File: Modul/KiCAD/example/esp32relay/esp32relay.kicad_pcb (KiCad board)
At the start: 2 copper layers, 49.7 x 53.8 mm, 22 parts, among them J1 Conn_01x03_Male, J2 Conn_01x02_Male, SW1 SW_Push, SW2 SW_Push, U1 ESP32-WROOM-32, U2 AMS1117-3.3

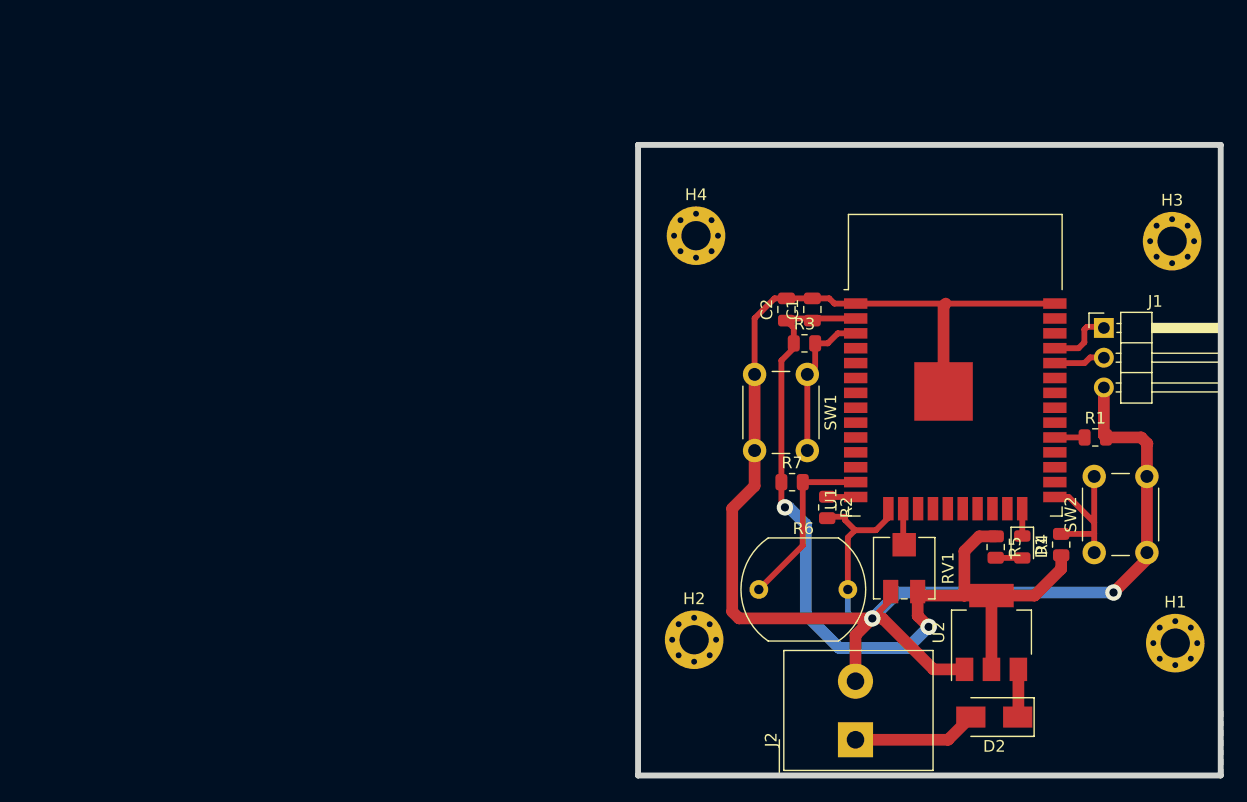
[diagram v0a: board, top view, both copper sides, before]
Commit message: KiCAD Fab Files
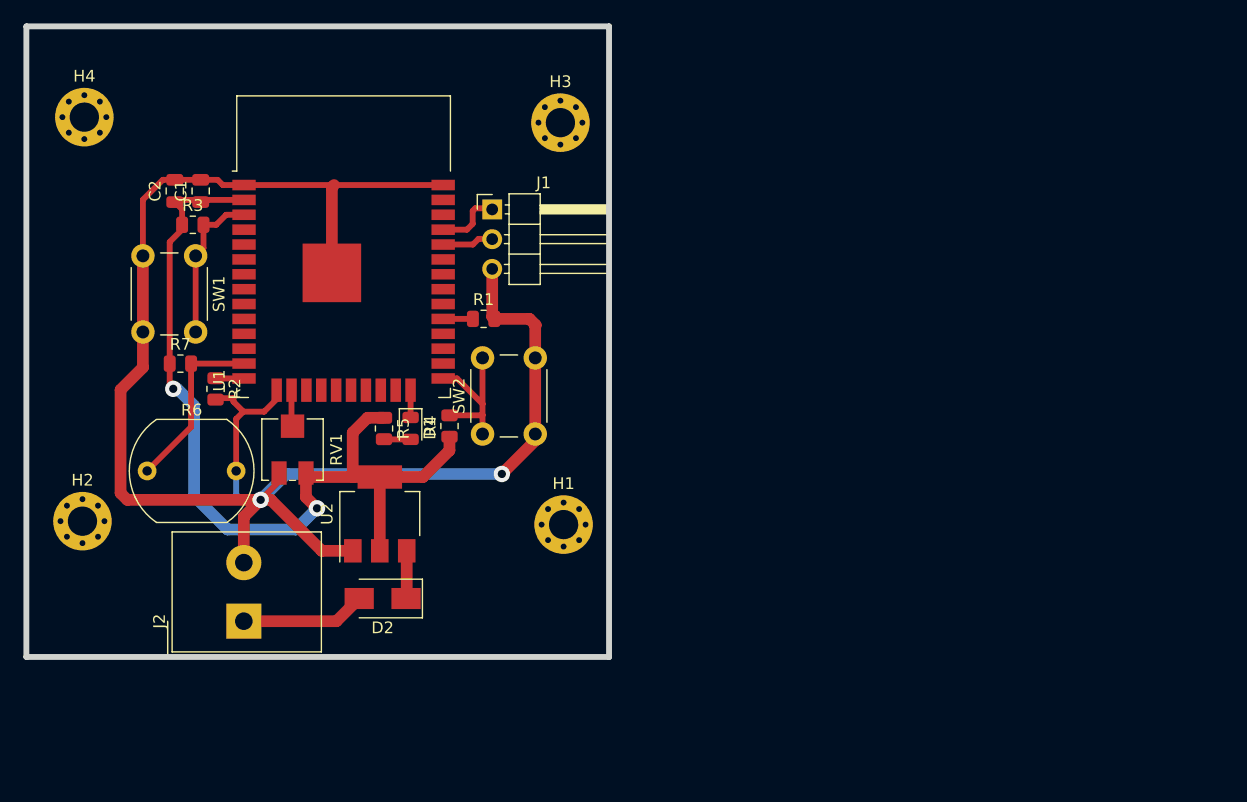
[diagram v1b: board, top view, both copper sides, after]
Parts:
- moved C2 53.2 mm to (34.4, 35.3)
- moved D1 53.2 mm to (54.6, 55.6)
- moved D2 53.2 mm to (52.2, 70.1)
- moved H1 53.2 mm to (67.6, 63.8)
- moved H4 53.2 mm to (26.7, 29.0)
- moved J1 53.2 mm to (61.5, 36.9)
- moved J2 53.2 mm to (40.3, 72.0)
- moved R1 53.2 mm to (60.8, 46.2)
- moved R3 53.2 mm to (36.0, 38.2)
- moved R5 53.2 mm to (52.3, 55.6)
- moved R6 53.2 mm to (32.1, 59.2)
- moved RV1 53.2 mm to (44.5, 57.4)
- moved SW1 53.2 mm to (36.2, 40.8)
- moved SW2 53.2 mm to (60.7, 56.0)
- moved U1 53.2 mm to (48.8, 43.0)
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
